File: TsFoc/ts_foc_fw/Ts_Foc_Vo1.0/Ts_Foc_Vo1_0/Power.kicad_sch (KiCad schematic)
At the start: 5 parts, among them Q1 JSM2301S

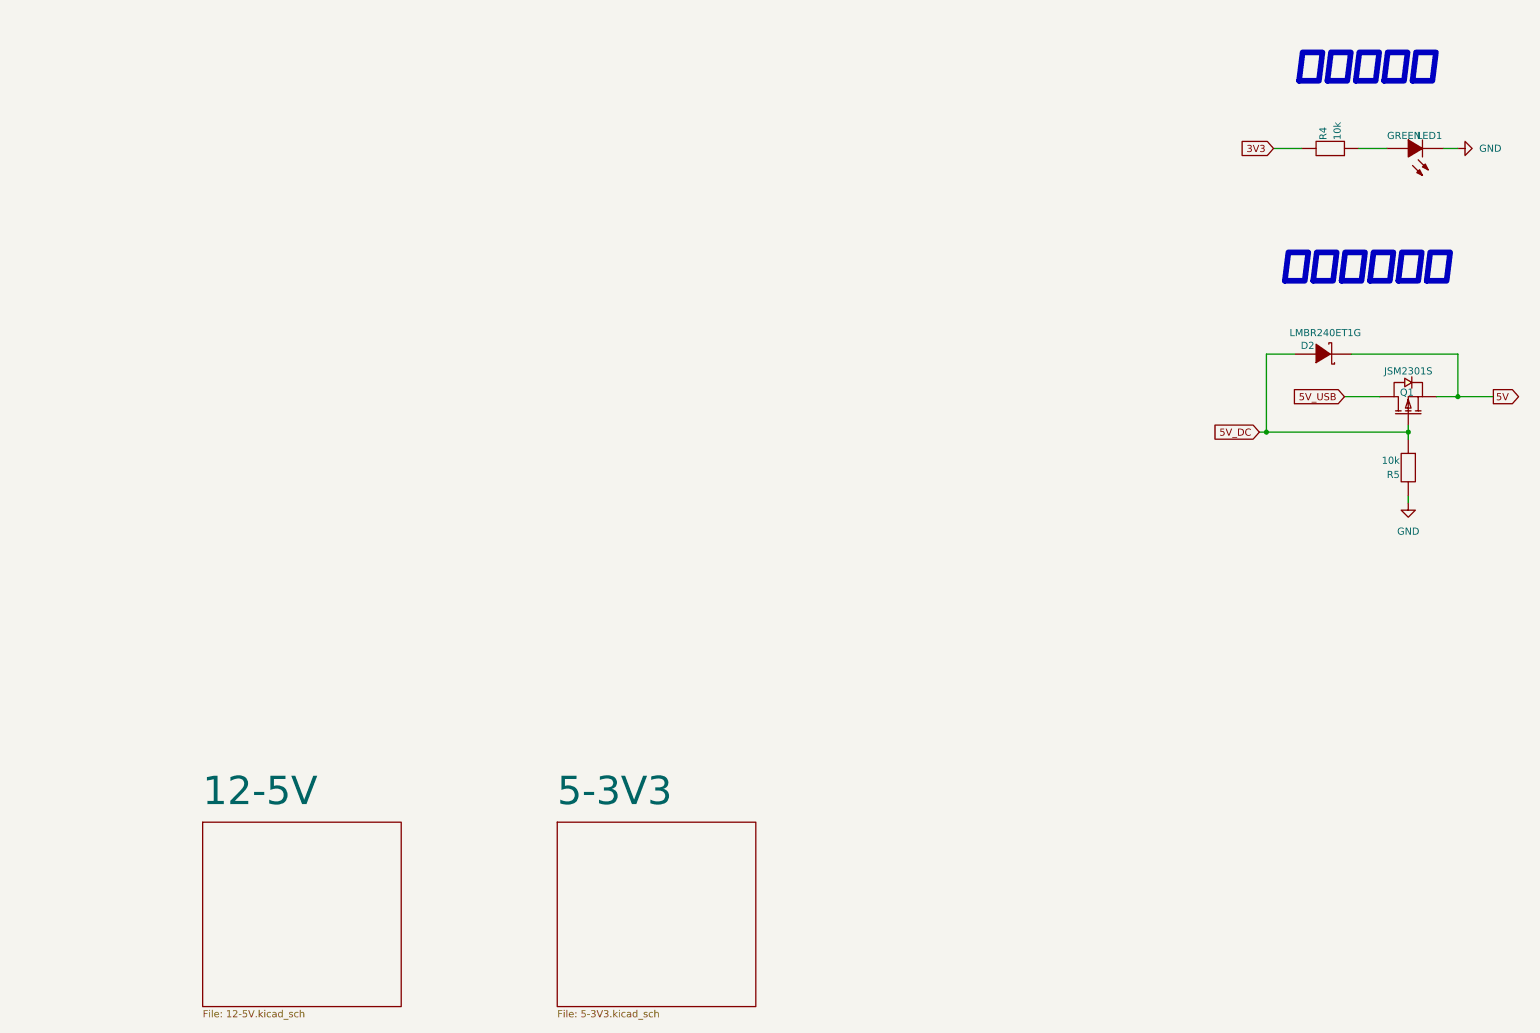
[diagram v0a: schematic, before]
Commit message: 同步_原理图小幅优化
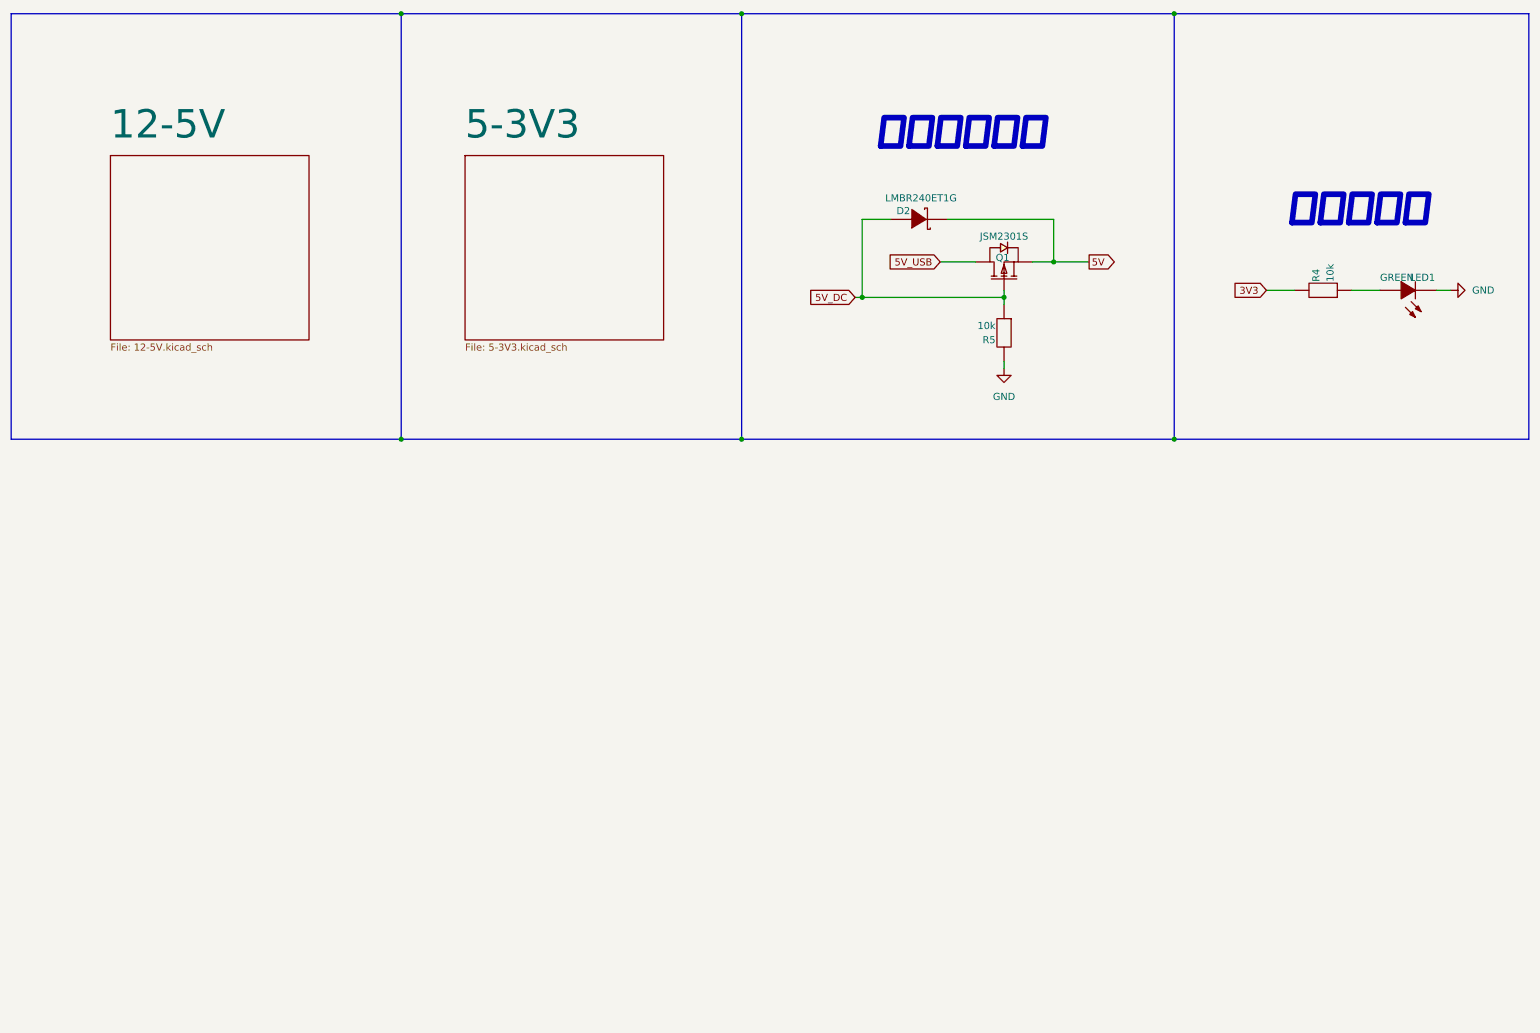
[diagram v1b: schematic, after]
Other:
- moved on the sheet: D2, LED1, Q1, R4, R5
